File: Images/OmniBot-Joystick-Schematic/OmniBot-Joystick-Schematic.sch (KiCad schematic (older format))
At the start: 9 parts

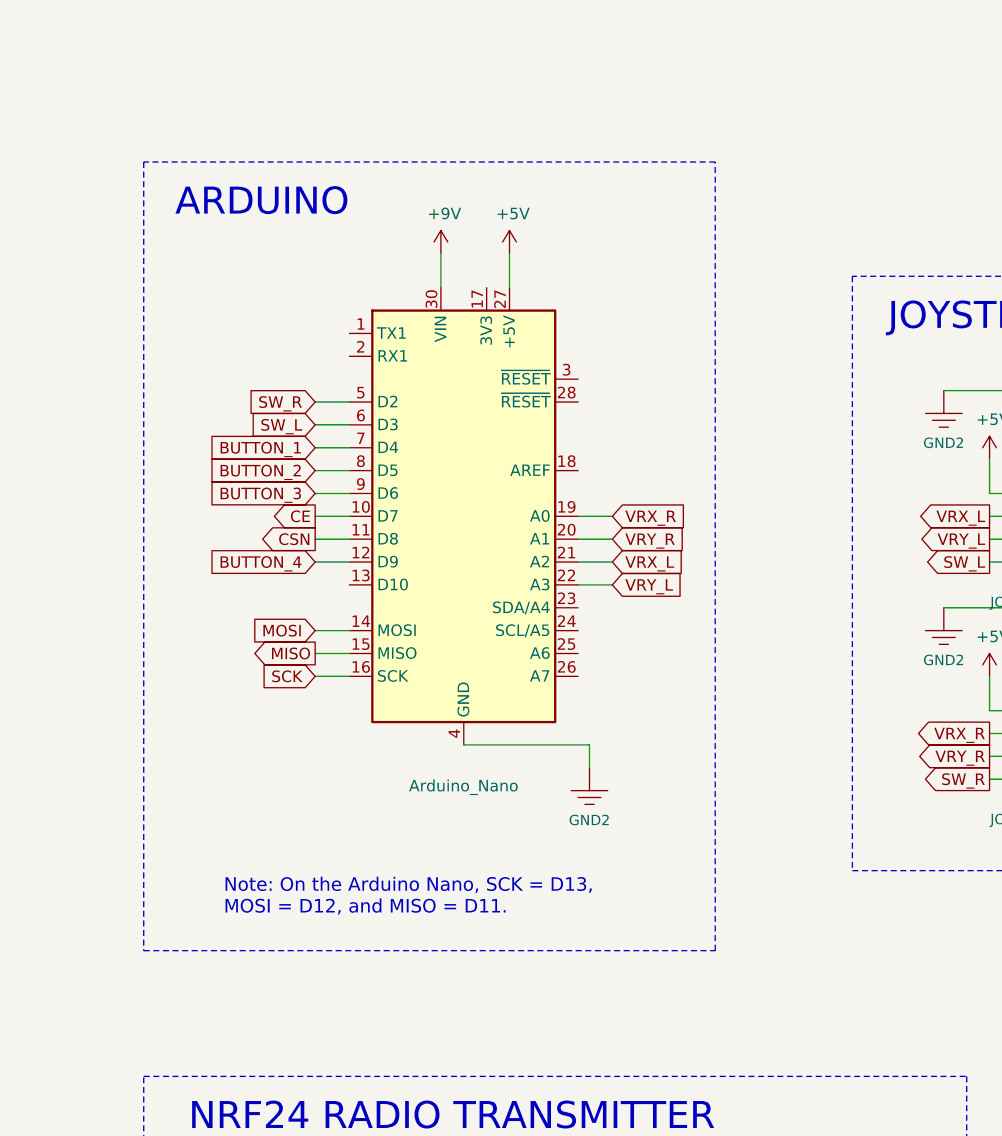
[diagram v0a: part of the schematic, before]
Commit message: Update schematic and code
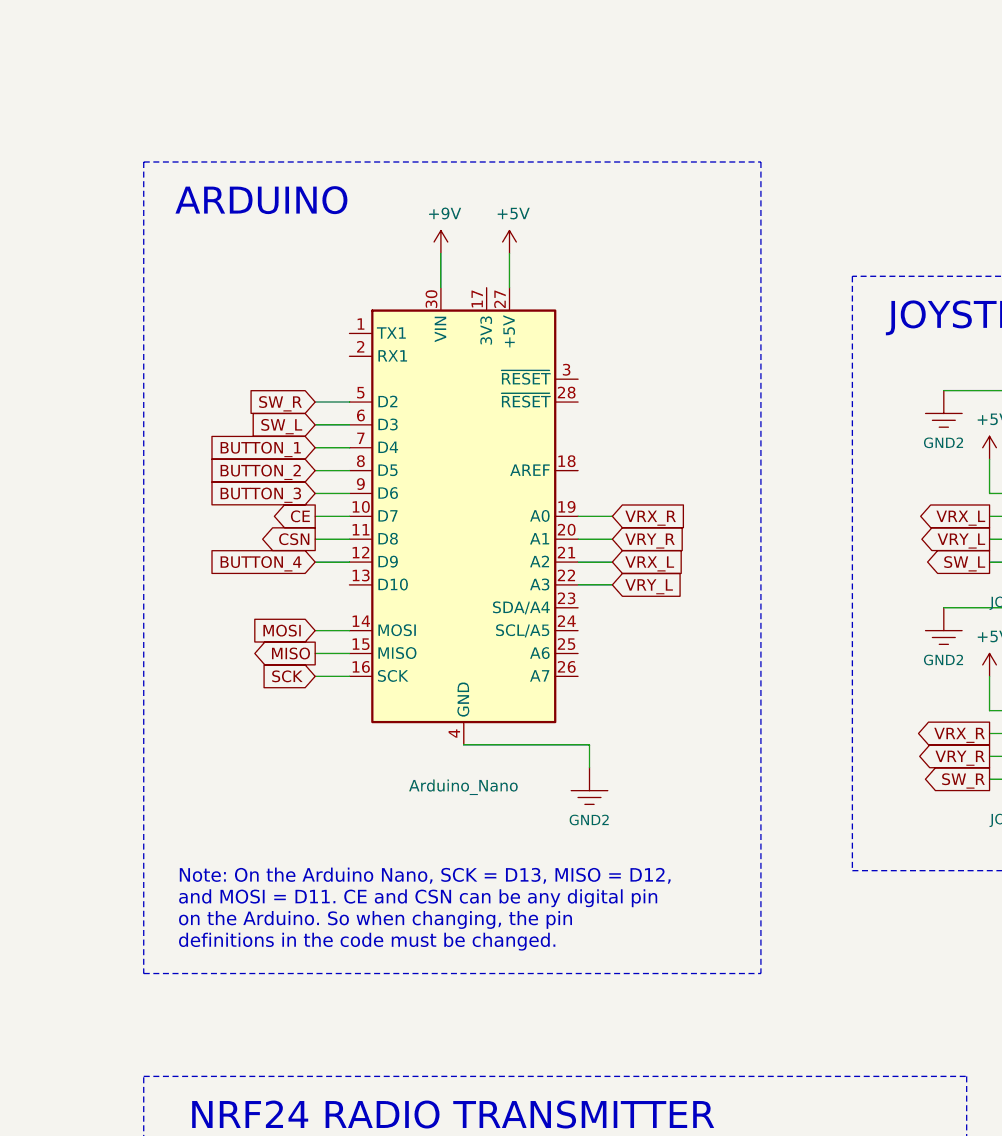
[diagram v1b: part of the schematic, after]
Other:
- note added: "Note: On the Arduino Nano, SCK = D13, MISO = D12, \nand MOSI = D11. CE and CSN can be any digital pin\non the Arduino. So when changing, the pin \ndefinitions in the code must be changed."
- note removed: "Note: On the Arduino Nano, SCK = D13, \nMOSI = D12, and MISO = D11."
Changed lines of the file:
@@
 Wire Notes Line
 	4500 2500 4500 5100
-Wire Notes Line
-	1400 5450 3900 5450
-Wire Notes Line
-	3900 5450 3900 2000
-Wire Notes Line
-	3900 2000 1400 2000
-Wire Notes Line
-	1400 2000 1400 5450
-Text Notes 1750 5300 0    59   ~ 0
-Note: On the Arduino Nano, SCK = D13, \nMOSI = D12, and MISO = D11.
+Text Notes 1550 5450 0    59   ~ 0
+Note: On the Arduino Nano, SCK = D13, MISO = D12, \nand MOSI = D11. CE and CSN can be any digital pin\non the Arduino. So when changing, the pin \ndefinitions in the code must be changed.
 $Comp
 L SparkFun-PowerSymbols:GND2 #GND?
@@
 Wire Wire Line
 	1750 6900 2650 6900
+Wire Notes Line
+	4100 2000 4100 5550
+Wire Notes Line
+	1400 2000 1400 5550
+Wire Notes Line
+	1400 5550 4100 5550
+Wire Notes Line
+	1400 2000 4100 2000
 $EndSCHEMATC
